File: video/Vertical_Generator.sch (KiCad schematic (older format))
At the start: 9 parts, among them U10 74LS08, U11 74LS08, U12 74LS163, U13 74LS163, U14 74LS163, U3 74LS08, U7 74LS08, U8 74LS04, U9 74LS02

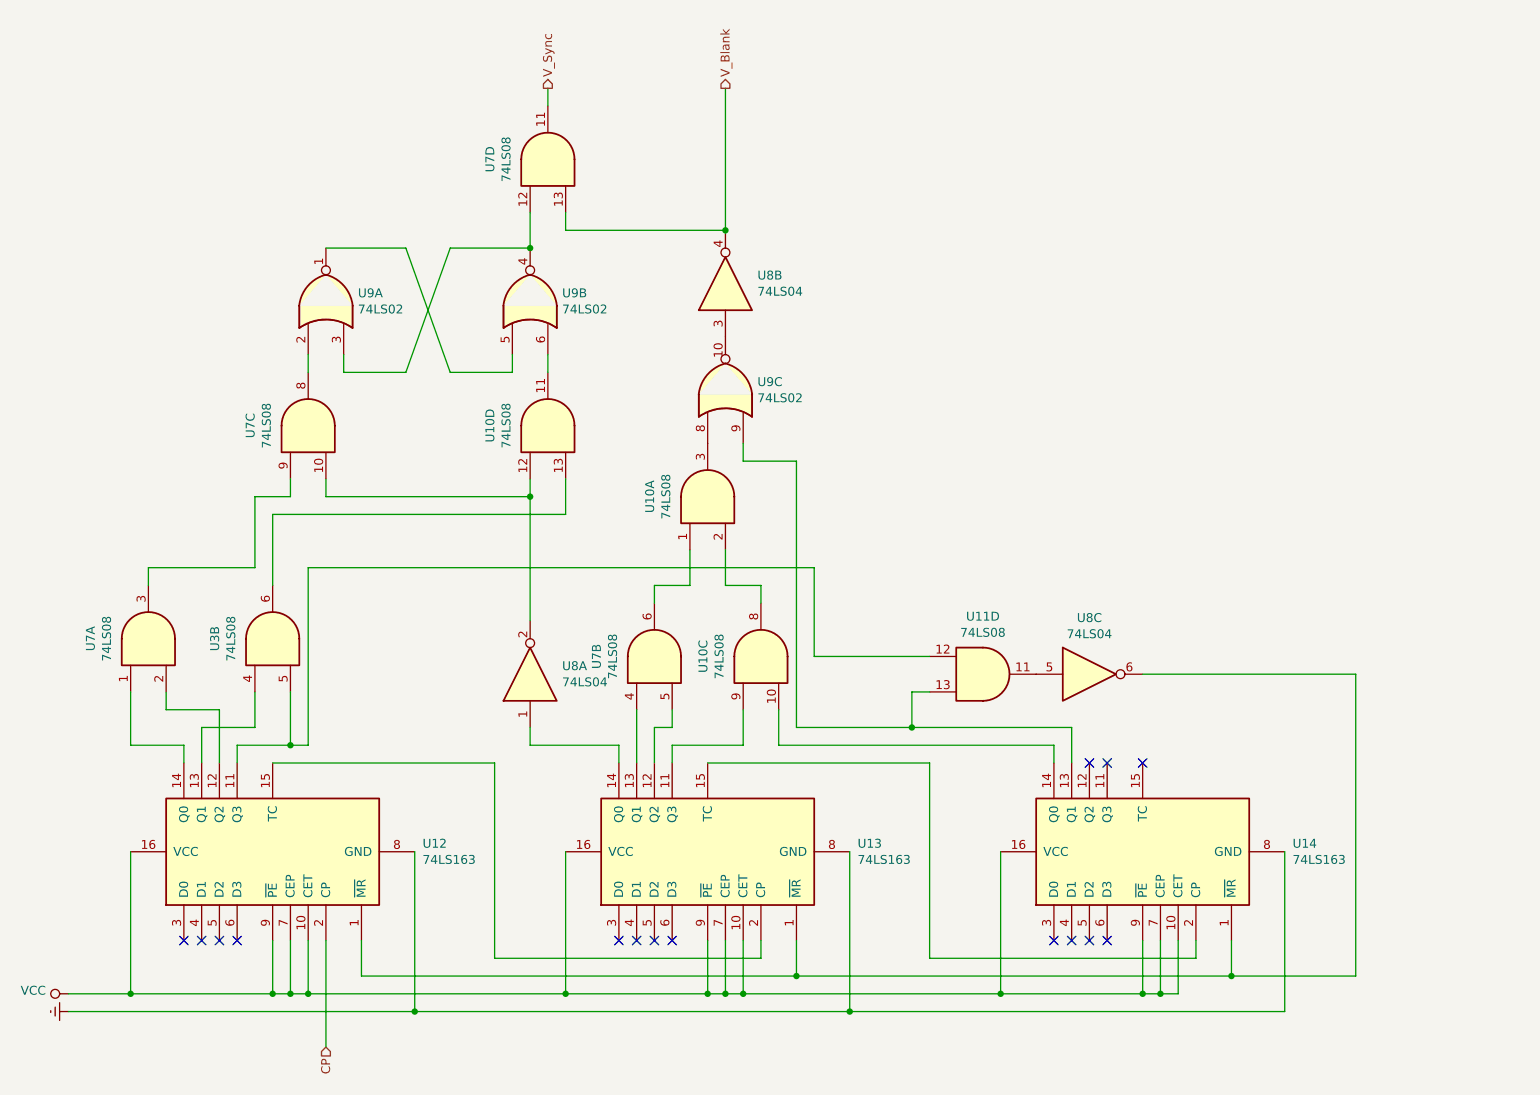
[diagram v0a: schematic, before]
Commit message: Resize and plot video
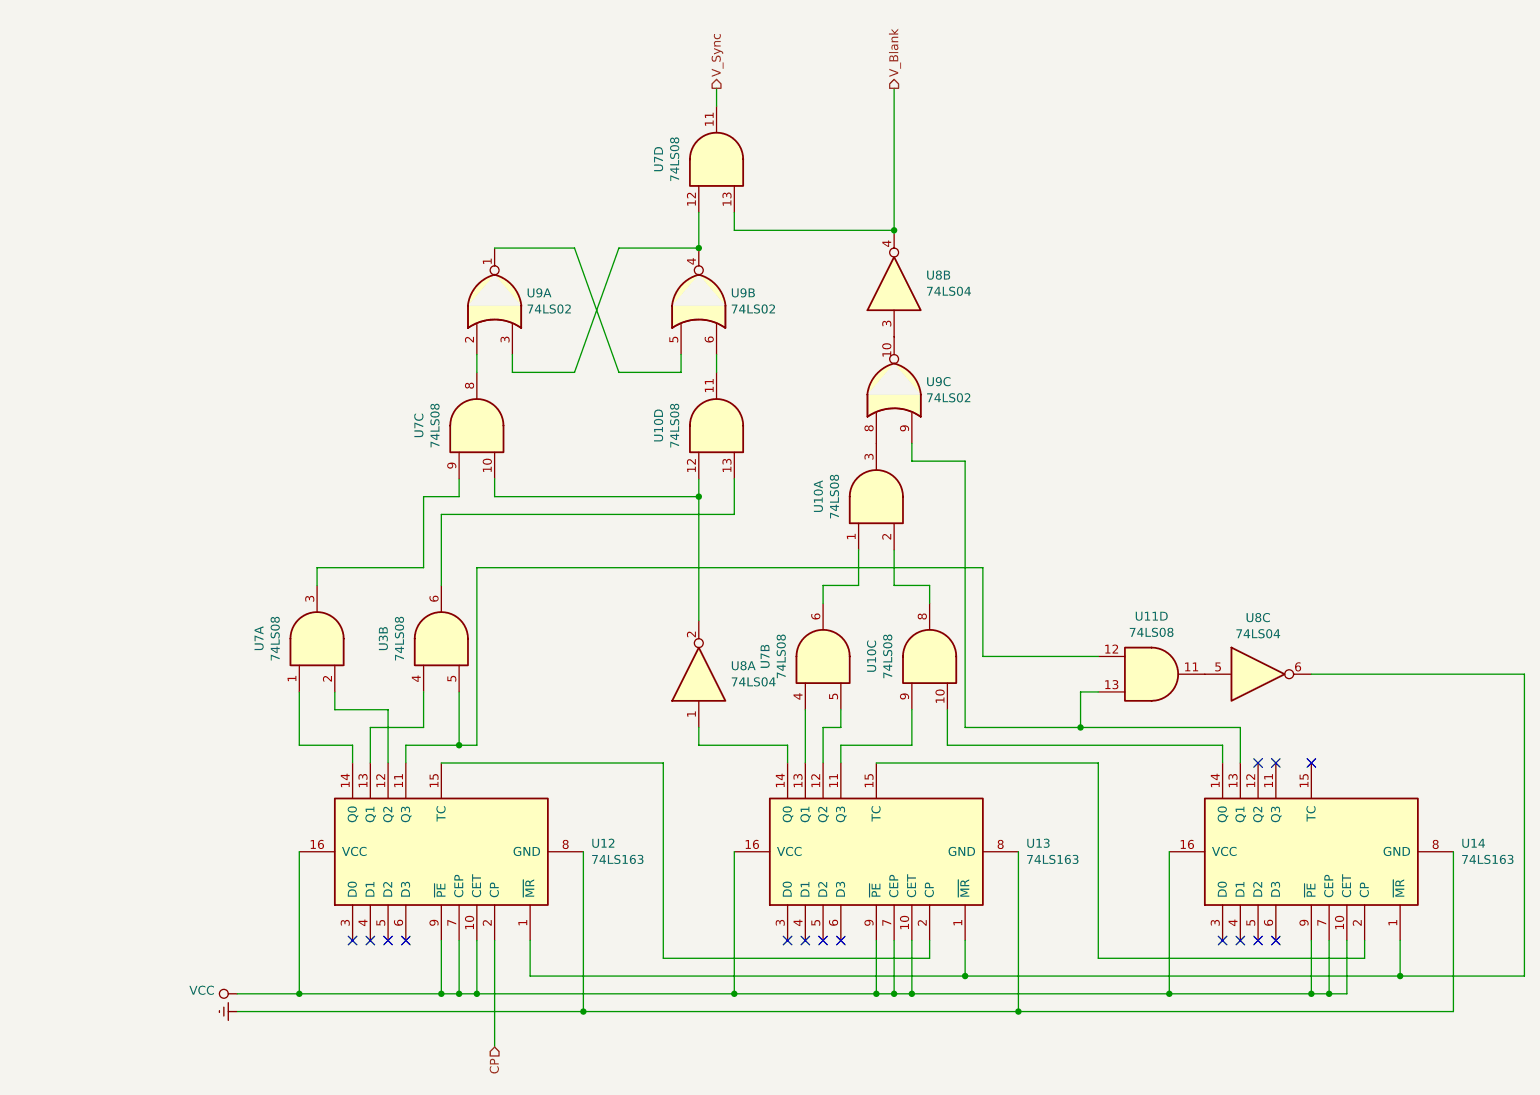
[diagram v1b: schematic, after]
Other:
- moved on the sheet: U10A, U10C, U10D, U11D, U12, U13, U14, U3B, U7A, U7B, U7C, U7D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
